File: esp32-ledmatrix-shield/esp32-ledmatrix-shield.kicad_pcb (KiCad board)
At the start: 2 copper layers, 91.4 x 62.2 mm, 22 parts, among them J1 Power, J10 C, J11 D, J12 E, J13 I2C, J14 I2C, J15 Power, J2 JIN, J3 Byp D1, J4 JOUT, J5 Power, J6 CON1 I2C2, J7 CON 2, J8 Buzzer, J9 I2C, U1 ESP32NODEMCU

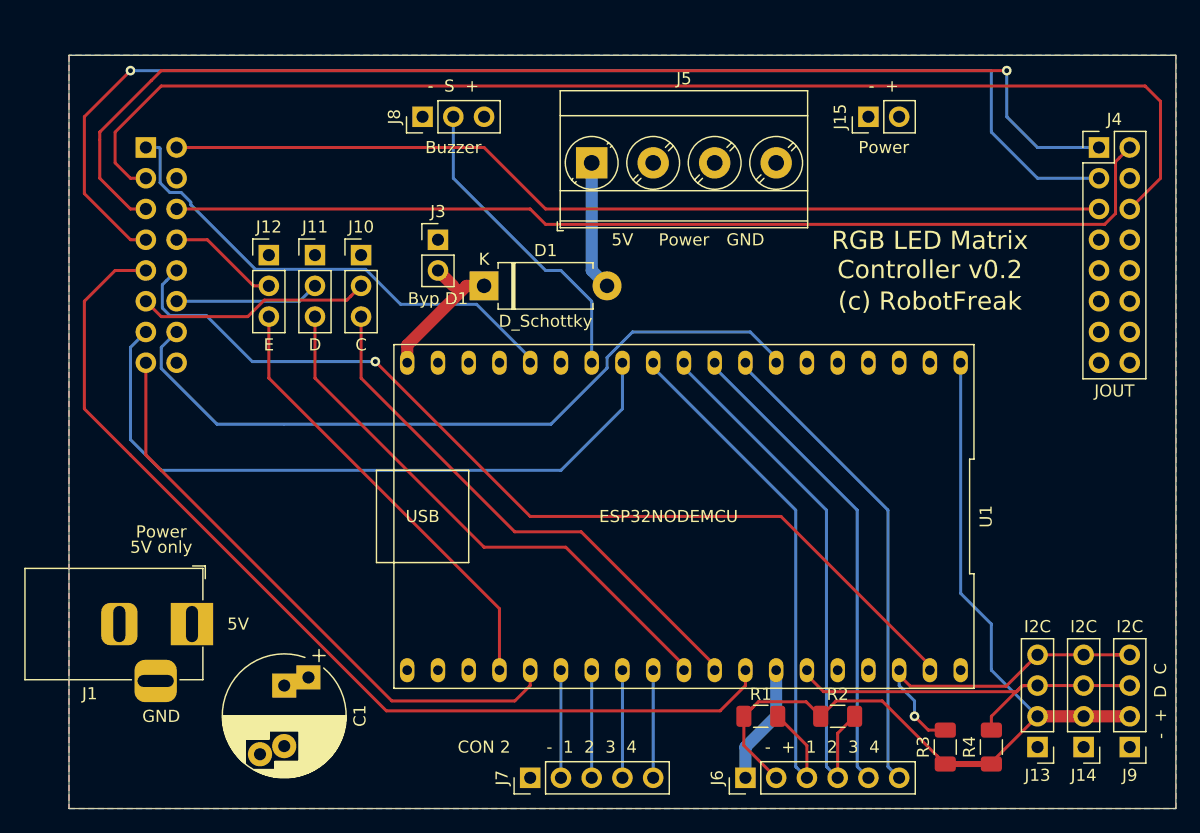
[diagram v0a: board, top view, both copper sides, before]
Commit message: schematic and pcb v0.3 devkit support
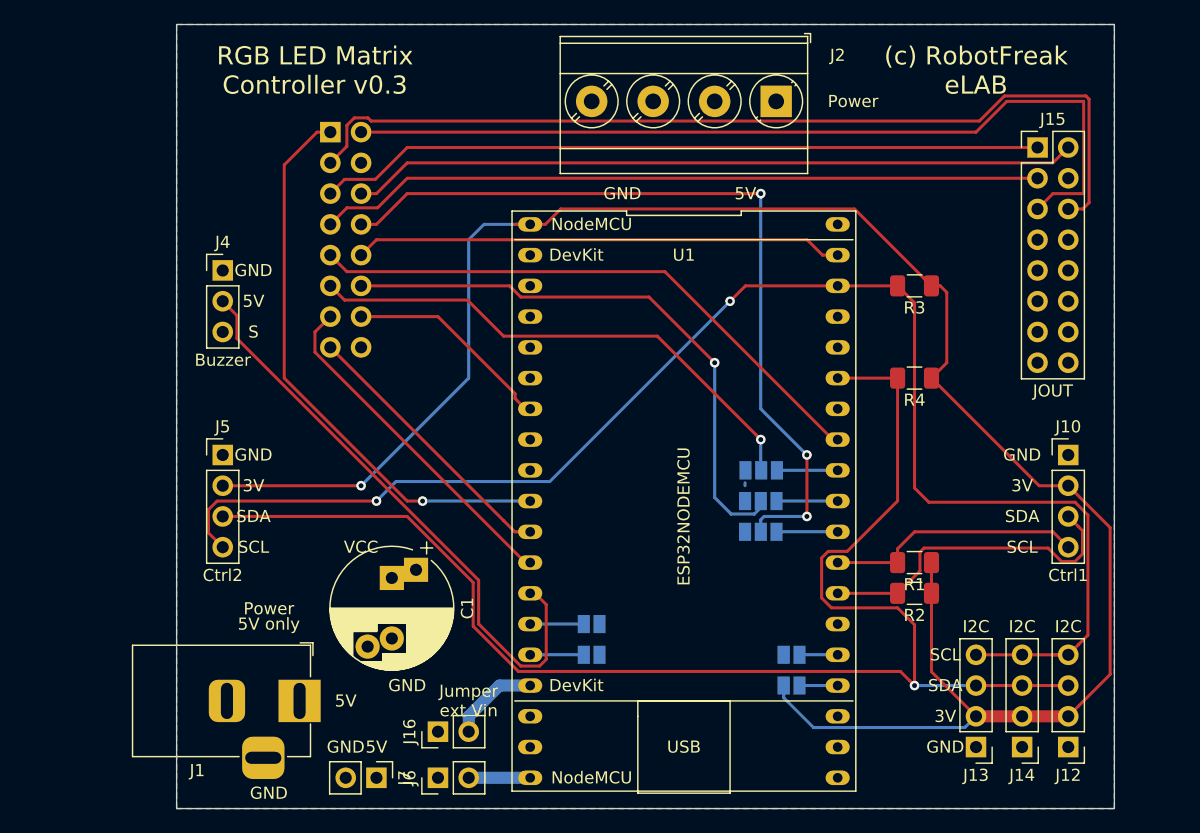
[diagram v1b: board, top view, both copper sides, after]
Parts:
- removed D1: D_Schottky, Diode_THT:D_DO-15_P10.16mm_Horizontal
- added J16: VIN ext, Connector_PinHeader_2.54mm:PinHeader_1x02_P2.54mm_Vertical, F.Cu at (124.5, 130.8)
- added JP1: Jumper, Jumper:SolderJumper-2_P1.3mm_Open_Pad1.0x1.5mm, B.Cu at (137.2, 121.9)
- added JP2: Jumper, Jumper:SolderJumper-2_P1.3mm_Open_Pad1.0x1.5mm, B.Cu at (137.2, 124.5)
- added JP3: Jumper, Jumper:SolderJumper-2_P1.3mm_Open_Pad1.0x1.5mm, B.Cu at (153.7, 124.5)
- added JP4: Jumper, Jumper:SolderJumper-2_P1.3mm_Open_Pad1.0x1.5mm, B.Cu at (153.7, 127.0)
- J10: value C -> Ctrl1; footprint Connector_PinHeader_2.54mm:PinHeader_1x03_P2.54mm_Vertical -> Connector_PinHeader_2.54mm:PinHeader_1x04_P2.54mm_Vertical
- J11: value D -> E; footprint Connector_PinHeader_2.54mm:PinHeader_1x03_P2.54mm_Vertical -> Jumper:SolderJumper-3_P1.3mm_Open_Pad1.0x1.5mm; moved to B.Cu
- J12: value E -> I2C; footprint Connector_PinHeader_2.54mm:PinHeader_1x03_P2.54mm_Vertical -> Connector_PinHeader_2.54mm:PinHeader_1x04_P2.54mm_Vertical
- J15: value Power -> JOUT; footprint Connector_PinHeader_2.54mm:PinHeader_1x02_P2.54mm_Vertical -> Connector_PinHeader_2.54mm:PinHeader_2x08_P2.54mm_Vertical
- J2: value JIN -> Power; footprint Connector_PinSocket_2.54mm:PinSocket_2x08_P2.54mm_Vertical -> TerminalBlock_Phoenix:TerminalBlock_Phoenix_MKDS-3-4-5.08_1x04_P5.08mm_Horizontal; moved to F.Cu
- J3: value Byp D1 -> JIN; footprint Connector_PinHeader_2.54mm:PinHeader_1x02_P2.54mm_Vertical -> Connector_PinSocket_2.54mm:PinSocket_2x08_P2.54mm_Vertical; moved to B.Cu
- J4: value JOUT -> Buzzer; footprint Connector_PinHeader_2.54mm:PinHeader_2x08_P2.54mm_Vertical -> Connector_PinHeader_2.54mm:PinHeader_1x03_P2.54mm_Vertical
- J5: value Power -> Ctrl2; footprint TerminalBlock_Phoenix:TerminalBlock_Phoenix_MKDS-3-4-5.08_1x04_P5.08mm_Horizontal -> Connector_PinHeader_2.54mm:PinHeader_1x04_P2.54mm_Vertical
- J6: value CON1 I2C2 -> VIN ext; footprint Connector_PinHeader_2.54mm:PinHeader_1x06_P2.54mm_Vertical -> Connector_PinHeader_2.54mm:PinHeader_1x02_P2.54mm_Vertical
- J7: value CON 2 -> Power; footprint Connector_PinHeader_2.54mm:PinHeader_1x05_P2.54mm_Vertical -> Connector_PinHeader_2.54mm:PinHeader_1x02_P2.54mm_Vertical
- J8: value Buzzer -> C; footprint Connector_PinHeader_2.54mm:PinHeader_1x03_P2.54mm_Vertical -> Jumper:SolderJumper-3_P1.3mm_Open_Pad1.0x1.5mm; moved to B.Cu
- J9: value I2C -> D; footprint Connector_PinHeader_2.54mm:PinHeader_1x04_P2.54mm_Vertical -> Jumper:SolderJumper-3_P1.3mm_Open_Pad1.0x1.5mm; moved to B.Cu
- moved J12 77.5 mm to (176.5, 132.1), turned to 180 degrees
- moved J4 73.1 mm to (106.7, 92.7)
- moved J10 60.7 mm to (176.5, 108.0)
- moved J2 52.2 mm to (152.4, 78.7)
- moved J11 43.3 mm to (151.1, 114.3)
- moved J8 40.4 mm to (151.2, 109.2), turned to 0 degrees
- moved J5 38.9 mm to (106.7, 108.0)
- moved R3 38.2 mm to (163.8, 94.0), turned to 180 degrees
- moved J9 36.6 mm to (151.1, 111.8), turned to 0 degrees
- moved R4 31.1 mm to (163.8, 101.6), turned to 180 degrees
- moved J6 25.4 mm to (124.5, 134.6)
- moved R1 18.0 mm to (163.8, 116.8), turned to 180 degrees
- moved J15 14.2 mm to (174.0, 82.5), turned to 0 degrees
- moved J7 12.7 mm to (119.4, 134.6), turned to 270 degrees
- moved C1 12.6 mm to (120.7, 118.1)
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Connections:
- J10 pad 2: /C -> +3V3
- J10 pad 3: Net-(J10-Pad3) -> /SDA2
- J11 pad 2: /D -> /E
- J12 pad 2: /E -> +3V3
- J12 pad 3: Net-(J12-Pad3) -> /SDA
- J13 pad 3: Net-(J13-Pad3) -> /SDA
- J13 pad 4: Net-(J13-Pad4) -> /SCL
- J14 pad 3: Net-(J13-Pad3) -> /SDA
- J14 pad 4: Net-(J13-Pad4) -> /SCL
- J15 pad 1: +5VA -> /R2
- J15 pad 2: GND -> /G2
- J2 pad 1: /R1 -> +5VA
- J2 pad 2: /G1 -> +5VA
- J2 pad 3: /B1 -> GND
- J3 pad 1: +5VA -> /R1
- J3 pad 2: Net-(D1-Pad1) -> /G1
- J4 pad 1: /R2 -> GND
- J4 pad 2: /G2 -> Net-(J4-Pad2)
- J4 pad 3: /B2 -> +5VA
- J5 pad 1: +5VA -> GND
- J5 pad 2: +5VA -> +3V3
- J5 pad 3: GND -> /SDA
- J5 pad 4: GND -> /SCL
- J6 pad 1: GND -> +5VA
- J6 pad 2: +3V3 -> Net-(J6-Pad2)
- J7 pad 1: GND -> +5VA
- J7 pad 2: Net-(J7-Pad2) -> GND
- J8 pad 2: Net-(J8-Pad2) -> /C
- J8 pad 3: +5VA -> /C'
- J9 pad 2: +3V3 -> /D
- J9 pad 3: Net-(J13-Pad3) -> Net-(J9-Pad3)
- R1 pad 2: Net-(J6-Pad3) -> /SCL2
- R2 pad 2: Net-(J6-Pad4) -> /SDA2
- R3 pad 2: Net-(J13-Pad4) -> /SCL
- R4 pad 2: Net-(J13-Pad3) -> /SDA
- U1 pad 10: Net-(J6-Pad4) -> /R1
- U1 pad 11: Net-(J6-Pad3) -> /OE
- U1 pad 13: Net-(J8-Pad2) -> Net-(J4-Pad2)
- U1 pad 14: GND -> Net-(JP1-Pad2)
- U1 pad 15: /R1 -> Net-(JP2-Pad2)
- U1 pad 19: Net-(D1-Pad1) -> Net-(J6-Pad2)
- U1 pad 23: Net-(J12-Pad3) -> Net-(JP4-Pad1)
- U1 pad 24: /OE -> Net-(JP3-Pad1)
- U1 pad 25: Net-(J7-Pad2) -> Net-(U1-Pad25)
- U1 pad 26: Net-(J7-Pad3) -> /SDA2
- U1 pad 27: Net-(J7-Pad4) -> /SCL2
- U1 pad 28: Net-(J7-Pad5) -> Net-(J11-Pad3)
- U1 pad 29: Net-(J11-Pad3) -> Net-(J9-Pad3)
- U1 pad 30: Net-(J10-Pad3) -> /C'
- U1 pad 32: GND -> Net-(U1-Pad32)
- U1 pad 33: Net-(J13-Pad3) -> /SDA
- U1 pad 36: Net-(J13-Pad4) -> /SCL
- U1 pad 8: Net-(J6-Pad6) -> Net-(U1-Pad8)
- U1 pad 9: Net-(J6-Pad5) -> Net-(U1-Pad9)
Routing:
- net /SCL: track 0.00 -> 122.2 mm, vias 0 -> 2
- net /SDA: track 0.00 -> 119.7 mm, vias 0 -> 1
- net +3V3: track 75.4 -> 165.8 mm, vias 0 -> 1
- net /E: track 9.20 -> 67.2 mm, vias 0 -> 3
- net Net-(J4-Pad2): track 0.00 -> 48.9 mm
- net Net-(J6-Pad3): track 45.6 -> 0.00 mm
- net Net-(J6-Pad4): track 45.2 -> 0.00 mm
- net /B2: track 105.1 -> 60.0 mm, vias 1 -> 0
- net Net-(J10-Pad3): track 44.5 -> 0.00 mm
- net /LAT: track 61.6 -> 17.4 mm
- net Net-(J11-Pad3): track 45.8 -> 5.30 mm
- net Net-(J6-Pad5): track 39.6 -> 0.00 mm
- net Net-(J6-Pad6): track 39.6 -> 0.00 mm
- net /B: track 79.6 -> 40.4 mm, vias 1 -> 0
- net /R2: track 98.2 -> 60.0 mm, vias 1 -> 0
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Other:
- board size 91.4 x 62.2 mm -> 77.5 x 64.8 mm
- board text added: "(c) RobotFreak eLAB"
- board text added: "3V"
- board text added: "DevKit"
- board text added: "Jumper ext Vin"
- board text added: "NodeMCU"
- board text added: "RGB LED Matrix Controller v0.3"
- board text added: "S"
- board text added: "SCL"
- board text added: "SDA"
- board text added: "VCC"
- board text removed: "(c) RobotFreak"
- board text removed: "- +"
- board text removed: "- + 1 2 3 4"
- board text removed: "- 1 2 3 4"
- board text removed: "- S +"
- board text removed: "RGB LED Matrix Controller v0.2"
